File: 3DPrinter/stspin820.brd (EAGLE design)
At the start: 127.6 x 42.2 mm, 19 parts, among them X1 CON-7.62-02P, X2 CON-XH-04

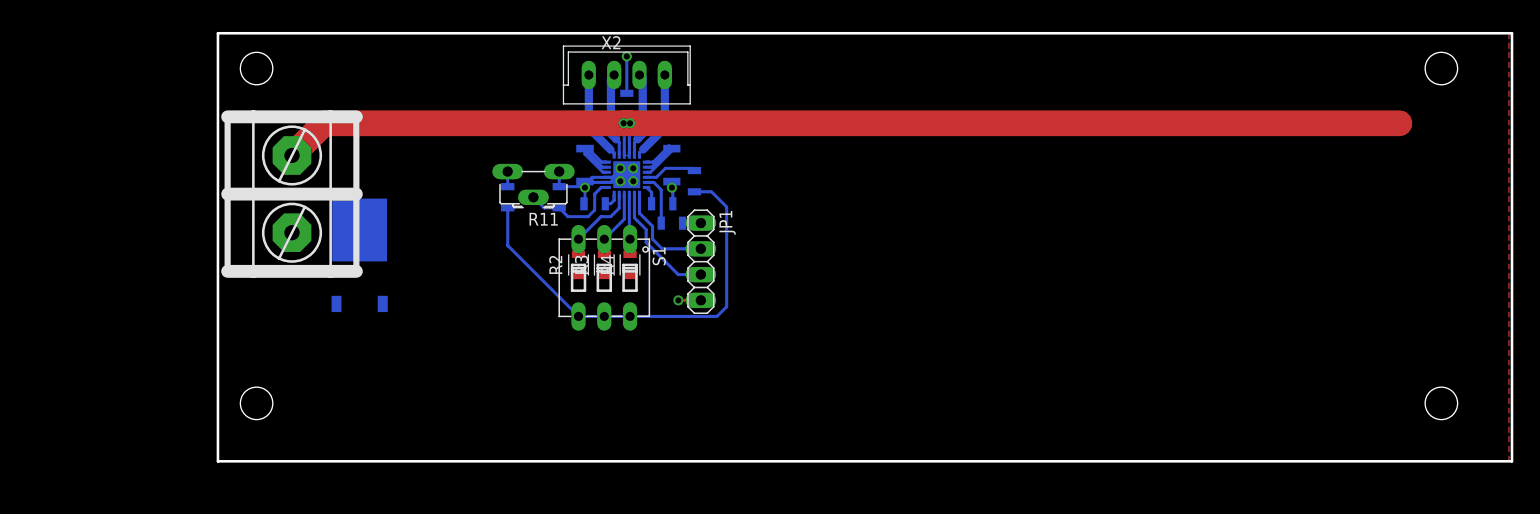
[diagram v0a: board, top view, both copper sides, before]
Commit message: Multiply
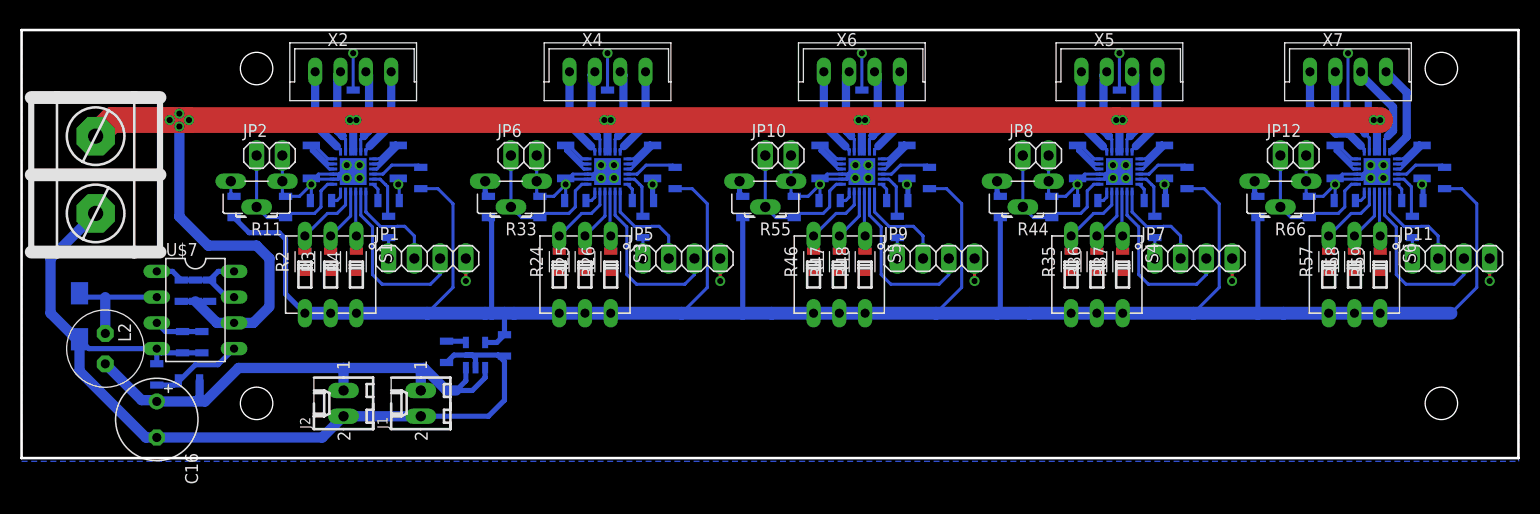
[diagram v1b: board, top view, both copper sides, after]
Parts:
- added C10, C11, C12, C4, C5, C6, C7, C8, C9: 1u, Flamberm:CAP0805
- added C14: 200p, Flamberm:CAP0805
- added C15: 68p, Flamberm:CAP0805
- added C16: (no value), Namenlos:E3,5-8
- added C3: 0u1, Flamberm:CAP0805
- added D2: (no value), Namenlos:DO214AC
- added J1, J2: 22-27-2021-02, con-molex:6410-02
- added JP10, JP12, JP2, JP6, JP8: (no value), pinhead:1X02
- added JP11, JP5, JP7, JP9: (no value), pinhead:1X04
- added L2: (no value), Namenlos:CW68
- added R12, R13, R14: 1R, Flamberm:RESC2012X50
- added R15: 1K5, Flamberm:RESC2012X50
- added R21: 13K, Flamberm:RESC2012X50
- added R23, R34, R45, R56: (no value), Flamberm:RESC2012X50
- added R24, R25, R26, R35, R36, R37, R46, R47, R48, R57, R58, R59: 20K, Flamberm:RESC2012X50
- added R27, R28, R38, R39, R49, R50, R60, R61: 0R43, Flamberm:RESC3216X60
- added R29, R30, R31, R40, R41, R42, R51, R52, R53, R62, R63, R64: 15K, Flamberm:RESC2012X50
- added R32, R43, R54, R65: 39K, Flamberm:RESC2012X50
- added R33, R44, R55, R66: (no value), pot:CA6H
- added S3, S4, S5, S6: (no value), Flamberm:DIP03YL
- added U$3, U$4, U$5, U$6: DRV-STSPIN820, Flamberm:QFN24
- added U$7: MC33063/MC34063P, adafruit:DIL08
- added X4, X5, X6, X7: CON-XH-04, Flamberm:XH-04
- U1: value (none) -> VREG-LD2985; device Flamberm:DPAK -> Flamberm:SOT95P280X145-5
- moved R1 27.9 mm to (16.8, 23.1), turned to 90 degrees
- moved R11 27.3 mm to (3.81, 27.6)
- moved C1 27.0 mm to (6.67, 25.1)
- moved R10 27.0 mm to (1.59, 25.1)
- moved R2 27.0 mm to (8.57, 19.7)
- moved JP1 27.0 mm to (20.6, 20.0), turned to 0 degrees
- moved R3 27.0 mm to (11.1, 19.7)
- moved R4 27.0 mm to (13.7, 19.7)
- moved R6 27.0 mm to (9.21, 29.5)
- moved R7 27.0 mm to (10.2, 25.7)
- moved R9 27.0 mm to (20.0, 27.9)
- moved S1 27.0 mm to (11.1, 18.4)
- moved C2 27.0 mm to (13.3, 35.6)
- moved R5 27.0 mm to (17.8, 29.5)
- moved R8 27.0 mm to (16.8, 25.7)
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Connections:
- removed net +5V: R10.1, R9.2, S1.4, S1.5, S1.6, U1.3
- new net +12V: C16.+, J1.1, J2.1, L2.P$2, R21.2, U1.1, U1.3
- new net +3V3: C4.1, R10.1, R31.2, R32.1, R42.2, R43.1, R53.2, R54.1, R64.2, R65.1, R9.2, S1.4, S1.5, S1.6, S3.4, S3.5, S3.6, S4.4, S4.5, S4.6, S5.4, S5.5, S5.6, S6.4, S6.5, S6.6, U1.5
- new net N$101: U$6.11, X7.3
- new net N$102: U$6.12, X7.4
- new net N$18: R32.2, R33.E
- new net N$19: R54.2, R55.E
- new net N$20: R43.2, R44.E
- new net N$21: R65.2, R66.E
- new net N$22: C14.1, C15.1, U$7.3
- new net N$23: R12.1, R13.1, R14.1, U$7.1, U$7.7, U$7.8
- new net N$24: D2.C, L2.P$1, U$7.2
- new net N$25: R15.1, R21.1, U$7.5
- new net N$26: C3.1, U1.4
- new net N$35: JP5.2, U$3.19
- new net N$36: JP5.3, U$3.20
- new net N$37: JP5.1, R23.1
- new net N$38: R23.2, U$3.17
- new net N$39: R26.2, S3.1, U$3.21
- new net N$40: R25.2, S3.2, U$3.22
- new net N$41: R24.2, S3.3, U$3.23
- new net N$42: R27.2, U$3.13, U$3.14, U$3.15
- new net N$43: R28.2, U$3.4, U$3.5, U$3.6
- new net N$44: U$3.7, X4.1
- new net N$45: U$3.8, X4.2
- new net N$46: R29.2, U$3.24
- new net N$47: R31.1, U$3.16
- new net N$48: R30.1, U$3.18
- new net N$50: U$3.11, X4.3
- new net N$51: U$3.12, X4.4
- new net N$52: JP7.2, U$4.19
- new net N$53: JP7.3, U$4.20
- new net N$54: JP7.1, R34.1
- new net N$55: R34.2, U$4.17
- new net N$56: R37.2, S4.1, U$4.21
- new net N$57: R36.2, S4.2, U$4.22
- new net N$58: R35.2, S4.3, U$4.23
- new net N$59: R38.2, U$4.13, U$4.14, U$4.15
- new net N$60: R39.2, U$4.4, U$4.5, U$4.6
- new net N$61: U$4.7, X5.1
- new net N$62: U$4.8, X5.2
- new net N$63: R40.2, U$4.24
- new net N$64: R42.1, U$4.16
- new net N$65: R41.1, U$4.18
- new net N$67: U$4.11, X5.3
- new net N$68: U$4.12, X5.4
- new net N$69: JP9.2, U$5.19
- new net N$70: JP9.3, U$5.20
- new net N$71: JP9.1, R45.1
- new net N$72: R45.2, U$5.17
- new net N$73: R48.2, S5.1, U$5.21
- new net N$74: R47.2, S5.2, U$5.22
- new net N$75: R46.2, S5.3, U$5.23
- new net N$76: R49.2, U$5.13, U$5.14, U$5.15
- new net N$77: R50.2, U$5.4, U$5.5, U$5.6
- new net N$78: U$5.7, X6.1
- new net N$79: U$5.8, X6.2
- new net N$80: R51.2, U$5.24
- new net N$81: R53.1, U$5.16
- new net N$82: R52.1, U$5.18
- new net N$84: U$5.11, X6.3
- new net N$85: U$5.12, X6.4
- new net N$86: JP11.2, U$6.19
- new net N$87: JP11.3, U$6.20
- new net N$88: JP11.1, R56.1
- new net N$89: R56.2, U$6.17
- new net N$90: R59.2, S6.1, U$6.21
- new net N$91: R58.2, S6.2, U$6.22
- new net N$92: R57.2, S6.3, U$6.23
- new net N$93: R60.2, U$6.13, U$6.14, U$6.15
- new net N$94: R61.2, U$6.4, U$6.5, U$6.6
- new net N$95: U$6.7, X7.1
- new net N$96: U$6.8, X7.2
- new net N$97: R62.2, U$6.24
- new net N$98: R64.1, U$6.16
- new net N$99: R63.1, U$6.18
- new net REF2: C5.1, JP6.1, R33.S, U$3.1
- new net REF3: C9.1, JP10.1, R55.S, U$5.1
- new net REF4: C7.1, JP8.1, R44.S, U$4.1
- new net REF5: C11.1, JP12.1, R66.S, U$6.1
- net +24V: now also C10.1, C12.1, C6.1, C8.1, R12.2, R13.2, R14.2, U$3.10, U$3.9, U$4.10, U$4.9, U$5.10, U$5.9, U$6.10, U$6.9, U$7.6; no longer U1.1
- net GND: now also C10.2, C11.2, C12.2, C14.2, C15.2, C16.-, C3.2, C4.2, C5.2, C6.2, C7.2, C8.2, C9.2, D2.A, J1.2, J2.2, JP10.2, JP11.4, JP12.2, JP2.2, JP5.4, JP6.2, JP7.4, JP8.2, JP9.4, R15.2, R24.1, R25.1, R26.1, R27.1, R28.1, R29.1, R30.2, R33.A, R35.1, R36.1, R37.1, R38.1, R39.1, R40.1, R41.2, R44.A, R46.1, R47.1, R48.1, R49.1, R50.1, R51.1, R52.2, R55.A, R57.1, R58.1, R59.1, R60.1, R61.1, R62.1, R63.2, R66.A, U$3.2, U$3.3, U$3.PAD, U$4.2, U$4.3, U$4.PAD, U$5.2, U$5.3, U$5.PAD, U$6.2, U$6.3, U$6.PAD, U$7.4, U1.2; no longer U1.2(PAD)
- net REF1: now also JP2.1
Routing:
- net +3V3: track 0.00 -> 248.5 mm
- net GND: track 22.5 -> 221.4 mm, vias 8 -> 40
- net +24V: track 119.4 -> 238.2 mm, vias 2 -> 14
- net +12V: track 0.00 -> 52.2 mm
- net +5V: track 42.2 -> 0.00 mm
- net N$87: track 0.00 -> 17.7 mm
- net N$70: track 0.00 -> 17.7 mm
- net N$36: track 0.00 -> 17.7 mm
- net N$53: track 0.00 -> 17.7 mm
- net REF4: track 0.00 -> 15.4 mm
- net REF2: track 0.00 -> 15.4 mm
- net REF3: track 0.00 -> 15.4 mm
- net REF5: track 0.00 -> 15.4 mm
- net N$23: track 0.00 -> 11.4 mm
- net N$24: track 0.00 -> 11.4 mm
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- added copper zone on layer 16, net GND
- removed copper zone on layer 16, net +24V
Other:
- board size 127.6 x 42.2 mm -> 147.6 x 42.2 mm

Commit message: Some Compacting
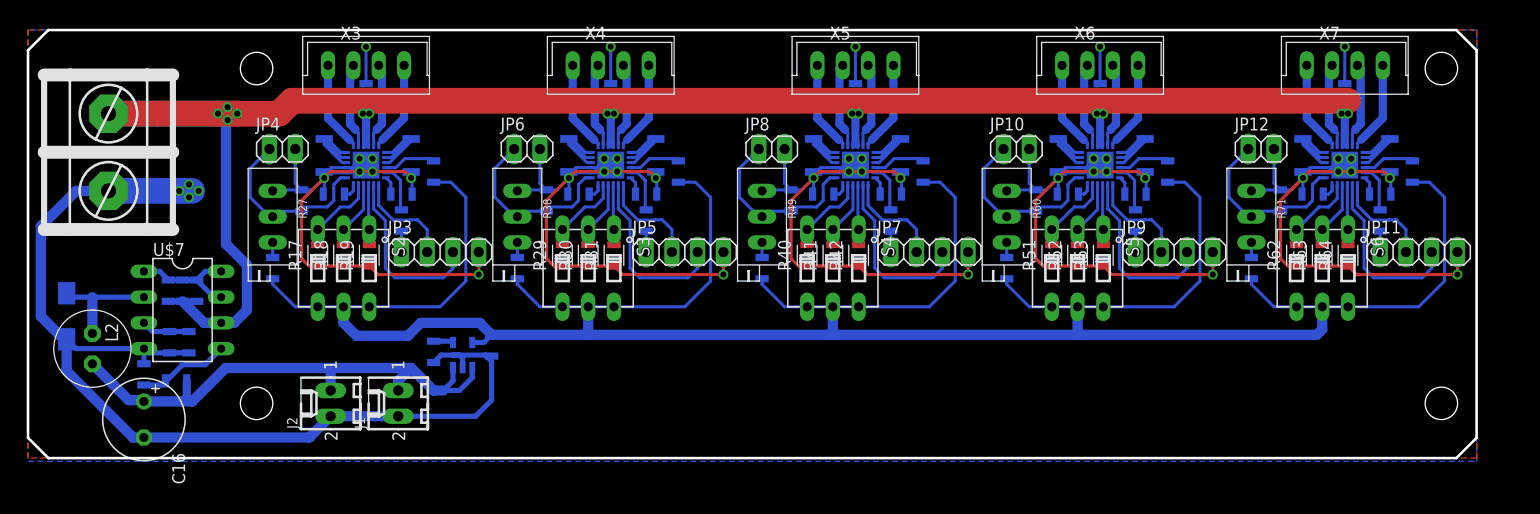
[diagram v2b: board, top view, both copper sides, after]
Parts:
- removed C1, C2: 1u, Flamberm:CAP0805
- removed JP1: (no value), pinhead:1X04
- removed JP2: (no value), pinhead:1X02
- removed R1: (no value), Flamberm:RESC2012X50
- removed R10: 39K, Flamberm:RESC2012X50
- removed R11: (no value), pot:CA6H
- removed R2, R3, R4: 20K, Flamberm:RESC2012X50
- removed R5, R6: 0R43, Flamberm:RESC3216X60
- removed R7, R8, R9: 15K, Flamberm:RESC2012X50
- removed S1: (no value), Flamberm:DIP03YL
- removed U$1: DRV-STSPIN820, Flamberm:QFN24
- removed X2: CON-XH-04, Flamberm:XH-04
- added C13, C17: 1u, Flamberm:CAP0805
- added JP3: (no value), pinhead:1X04
- added JP4: (no value), pinhead:1X02
- added R16: (no value), Flamberm:RESC2012X50
- added R17, R18, R19: 20K, Flamberm:RESC2012X50
- added R20, R22: 0R43, Flamberm:RESC3216X60
- added R67, R68, R69: 15K, Flamberm:RESC2012X50
- added R70: 39K, Flamberm:RESC2012X50
- added R71: (no value), Flamberm:POT-3296X
- added S2: (no value), Flamberm:DIP03YL
- added U$2: DRV-STSPIN820, Flamberm:QFN24
- added X3: CON-XH-04, Flamberm:XH-04
- R23, R34, R45, R56: value (none) -> 15K
- R24, R25, R35, R36, R46, R47, R57, R58: value 20K -> 15K
- R26, R37, R48, R59: value 20K -> 39K
- R27, R38, R49, R60: value 0R43 -> (none); device Flamberm:RESC3216X60 -> Flamberm:POT-3296X
- R28, R39, R50, R61: value 0R43 -> (none); device Flamberm:RESC3216X60 -> Flamberm:RESC2012X50
- R29, R30, R31, R40, R41, R42, R51, R52, R53, R62, R63, R64: value 15K -> 20K
- R32, R43, R54, R65: value 39K -> 0R43; device Flamberm:RESC2012X50 -> Flamberm:RESC3216X60
- R33, R44, R55, R66: value (none) -> 0R43; device pot:CA6H -> Flamberm:RESC3216X60
- moved R38 64.0 mm to (29.5, 24.1), flipped to the top, turned to 180 degrees
- moved R37 59.7 mm to (29.5, 19.1), flipped to the bottom
- moved R34 56.9 mm to (35.6, 26.4), turned to 180 degrees
- moved C8 50.2 mm to (38.7, 36.2)
- moved C7 49.9 mm to (32.4, 25.7)
- moved R35 42.4 mm to (42.2, 26.4), flipped to the bottom, turned to 180 degrees
- moved R36 42.2 mm to (45.4, 28.6), flipped to the bottom, turned to 270 degrees
- moved R60 41.3 mm to (77.8, 24.1), flipped to the top, turned to 180 degrees
- moved R54 40.0 mm to (91.4, 30.2)
- moved R27 37.9 mm to (5.40, 24.1), flipped to the top, turned to 180 degrees
- moved R59 36.8 mm to (77.8, 19.1), flipped to the bottom
- moved R56 34.1 mm to (83.8, 26.4), turned to 180 degrees
- moved R26 33.3 mm to (5.40, 19.1), flipped to the bottom
- moved R42 33.3 mm to (63.2, 20.3), flipped to the top, turned to 90 degrees
- moved R41 32.2 mm to (60.6, 20.3), flipped to the top, turned to 90 degrees
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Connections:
- removed net N$1: U$1.7, X2.1
- removed net N$10: R5.2, U$1.13, U$1.14, U$1.15
- removed net N$11: R6.2, U$1.4, U$1.5, U$1.6
- removed net N$12: U$1.11, X2.3
- removed net N$13: U$1.12, X2.4
- removed net N$14: R7.2, U$1.24
- removed net N$15: R9.1, U$1.16
- removed net N$16: R8.1, U$1.18
- removed net N$17: R10.2, R11.E
- removed net N$18: R32.2, R33.E
- removed net N$2: JP1.1, R1.1
- removed net N$3: JP1.2, U$1.19
- removed net N$38: R23.2, U$3.17
- removed net N$4: JP1.3, U$1.20
- removed net N$42 (its old number): R27.2, U$3.13, U$3.14, U$3.15
- removed net N$43 (its old number): R28.2, U$3.4, U$3.5, U$3.6
- removed net N$5: R1.2, U$1.17
- removed net N$57: R36.2, S4.2, U$4.22
- removed net N$58 (its old number): R35.2, S4.3, U$4.23
- removed net N$59 (its old number): R38.2, U$4.13, U$4.14, U$4.15
- removed net N$6: R4.2, S1.1, U$1.21
- removed net N$7: R3.2, S1.2, U$1.22
- removed net N$71 (its old number): JP9.1, R45.1
- removed net N$72 (its old number): R45.2, U$5.17
- removed net N$76: R49.2, U$5.13, U$5.14, U$5.15
- removed net N$77 (its old number): R50.2, U$5.4, U$5.5, U$5.6
- removed net N$8: R2.2, S1.3, U$1.23
- removed net N$80 (its old number): R51.2, U$5.24
- removed net N$81 (its old number): R53.1, U$5.16
- removed net N$9: U$1.8, X2.2
- removed net N$90 (its old number): R59.2, S6.1, U$6.21
- removed net N$91 (its old number): R58.2, S6.2, U$6.22
- removed net N$97 (its old number): R62.2, U$6.24
- removed net N$99 (its old number): R63.1, U$6.18
- new net N$102: JP11.1, R61.1
- new net N$103: R61.2, U$6.17
- new net N$104: R64.2, S6.1, U$6.21
- new net N$105: R63.2, S6.2, U$6.22
- new net N$106: R62.2, S6.3, U$6.23
- new net N$107: R65.2, U$6.13, U$6.14, U$6.15
- new net N$108: R66.2, U$6.4, U$6.5, U$6.6
- new net N$111: R67.2, U$6.24
- new net N$112: R69.1, U$6.16
- new net N$113: R68.1, U$6.18
- new net N$117: R70.2, R71.3
- new net N$27: R16.2, U$2.17
- new net N$28: R19.2, S2.1, U$2.21
- new net N$29: R18.2, S2.2, U$2.22
- new net N$30: R17.2, S2.3, U$2.23
- new net N$31: R20.2, U$2.13, U$2.14, U$2.15
- new net N$32: R22.2, U$2.4, U$2.5, U$2.6
- new net N$33: U$2.7, X3.1
- new net N$34: U$2.8, X3.2
- new net N$35: R23.2, U$2.24
- new net N$36: R25.1, U$2.16
- new net N$44: JP5.1, R28.1
- new net N$45: R28.2, U$3.17
- new net N$50: R32.2, U$3.13, U$3.14, U$3.15
- new net N$51: R33.2, U$3.4, U$3.5, U$3.6
- new net N$67: R41.2, S4.2, U$4.22
- new net N$68: R40.2, S4.3, U$4.23
- new net N$69: R43.2, U$4.13, U$4.14, U$4.15
- new net N$70: R44.2, U$4.4, U$4.5, U$4.6
- new net N$79: R48.2, R49.3
- new net N$84: R50.2, U$5.17
- new net N$85: R53.2, S5.1, U$5.21
- new net N$86: R52.2, S5.2, U$5.22
- new net N$87: R51.2, S5.3, U$5.23
- net +24V: now also C17.1, U$2.10, U$2.9; no longer C2.1, U$1.10, U$1.9
- net +3V3: now also R25.2, R26.1, R36.2, R37.1, R47.2, R48.1, R58.2, R59.1, R69.2, R70.1, S2.4, S2.5, S2.6; no longer R10.1, R31.2, R32.1, R42.2, R43.1, R53.2, R54.1, R64.2, R65.1, R9.2, S1.4, S1.5, S1.6
- net GND: now also C13.2, C17.2, JP3.4, JP4.2, R17.1, R18.1, R19.1, R20.1, R22.1, R23.1, R24.2, R30.1, R31.1, R32.1, R33.1, R34.1, R35.2, R41.1, R42.1, R43.1, R44.1, R45.1, R46.2, R52.1, R53.1, R54.1, R55.1, R56.1, R57.2, R63.1, R64.1, R65.1, R66.1, R67.1, R68.2, R71.1, U$2.2, U$2.3, U$2.PAD; no longer C1.2, C2.2, JP1.4, JP2.2, R11.A, R2.1, R24.1, R25.1, R26.1, R28.1, R3.1, R30.2, R33.A, R35.1, R36.1, R37.1, R39.1, R4.1, R41.2, R44.A, R46.1, R47.1, R48.1, R5.1, R50.1, R52.2, R55.A, R57.1, R58.1, R59.1, R6.1, R61.1, R63.2, R66.A, R7.1, R8.2, U$1.2, U$1.3, U$1.PAD
- net N$19: now also JP3.2, U$2.19; no longer R54.2, R55.E
- net N$20: now also JP3.3, U$2.20; no longer R43.2, R44.E
- net N$21: now also JP3.1, R16.1; no longer R65.2, R66.E
- net N$37: now also R24.1, U$2.18; no longer JP5.1, R23.1
- net N$39: now also U$2.11, X3.3; no longer R26.2, S3.1, U$3.21
- net N$40: now also U$2.12, X3.4; no longer R25.2, S3.2, U$3.22
- net N$41: now also R26.2, R27.3; no longer R24.2, S3.3, U$3.23
- net N$46: now also R31.2, S3.1, U$3.21; no longer R29.2, U$3.24
- net N$47: now also R30.2, S3.2, U$3.22; no longer R31.1, U$3.16
- net N$48: now also R29.2, S3.3, U$3.23; no longer R30.1, U$3.18
- net N$54: now also R34.2, U$3.24; no longer JP7.1, R34.1
- net N$55: now also R36.1, U$3.16; no longer R34.2, U$4.17
- net N$56: now also R35.1, U$3.18; no longer R37.2, S4.1, U$4.21
- net N$60: now also R37.2, R38.3; no longer R39.2, U$4.4, U$4.5, U$4.6
- net N$63: now also JP7.1, R39.1; no longer R40.2, U$4.24
- net N$64: now also R39.2, U$4.17; no longer R42.1, U$4.16
- net N$65: now also R42.2, S4.1, U$4.21; no longer R41.1, U$4.18
- net N$73: now also R45.2, U$4.24; no longer R48.2, S5.1, U$5.21
- net N$74: now also R47.1, U$4.16; no longer R47.2, S5.2, U$5.22
- net N$75: now also R46.1, U$4.18; no longer R46.2, S5.3, U$5.23
- net N$82: now also JP9.1, R50.1; no longer R52.1, U$5.18
- net N$88: now also R54.2, U$5.13, U$5.14, U$5.15; no longer JP11.1, R56.1
- net N$89: now also R55.2, U$5.4, U$5.5, U$5.6; no longer R56.2, U$6.17
- net N$92: now also R56.2, U$5.24; no longer R57.2, S6.3, U$6.23
- net N$93: now also R58.1, U$5.16; no longer R60.2, U$6.13, U$6.14, U$6.15
- net N$94: now also R57.1, U$5.18; no longer R61.2, U$6.4, U$6.5, U$6.6
- net N$98: now also R59.2, R60.3; no longer R64.1, U$6.16
- net REF1: now also C5.1, JP4.1, R27.2, U$2.1; no longer C1.1, JP2.1, R11.S, U$1.1
- net REF2: now also C7.1, R38.2; no longer C5.1, R33.S
- net REF3: now also JP8.1, R49.2, U$4.1; no longer JP10.1, R55.S, U$5.1
- net REF4: now also C11.1, JP10.1, R60.2, U$5.1; no longer C7.1, JP8.1, R44.S, U$4.1
- net REF5: now also C13.1, R71.2; no longer C11.1, R66.S
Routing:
- net GND: track 221.4 -> 435.8 mm, vias 40 -> 44
- net +3V3: track 248.5 -> 280.6 mm
- net N$4: track 17.7 -> 0.00 mm
- net N$20: track 1.62 -> 17.7 mm
- net N$59 (its old number): track 10.2 -> 0.00 mm
- net N$69: track 0.00 -> 10.2 mm
- net N$10: track 10.2 -> 0.00 mm
- net N$31: track 0.00 -> 10.2 mm
- net N$42 (its old number): track 10.2 -> 0.00 mm
- net N$50: track 0.00 -> 10.2 mm
- net N$76: track 10.2 -> 0.00 mm
- net N$107: track 0.00 -> 10.2 mm
- net N$3: track 10.0 -> 0.00 mm
- net +24V: track 238.2 -> 247.7 mm
- net N$43 (its old number): track 9.33 -> 0.00 mm
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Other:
- board size 147.6 x 42.2 mm -> 142.9 x 42.2 mm
